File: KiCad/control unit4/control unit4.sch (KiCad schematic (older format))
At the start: 38 parts, among them J1 Conn_01x02_Female, J2 Conn_01x03_Female, J5 Conn_01x02_Female, U1 LM358, U2 LM358

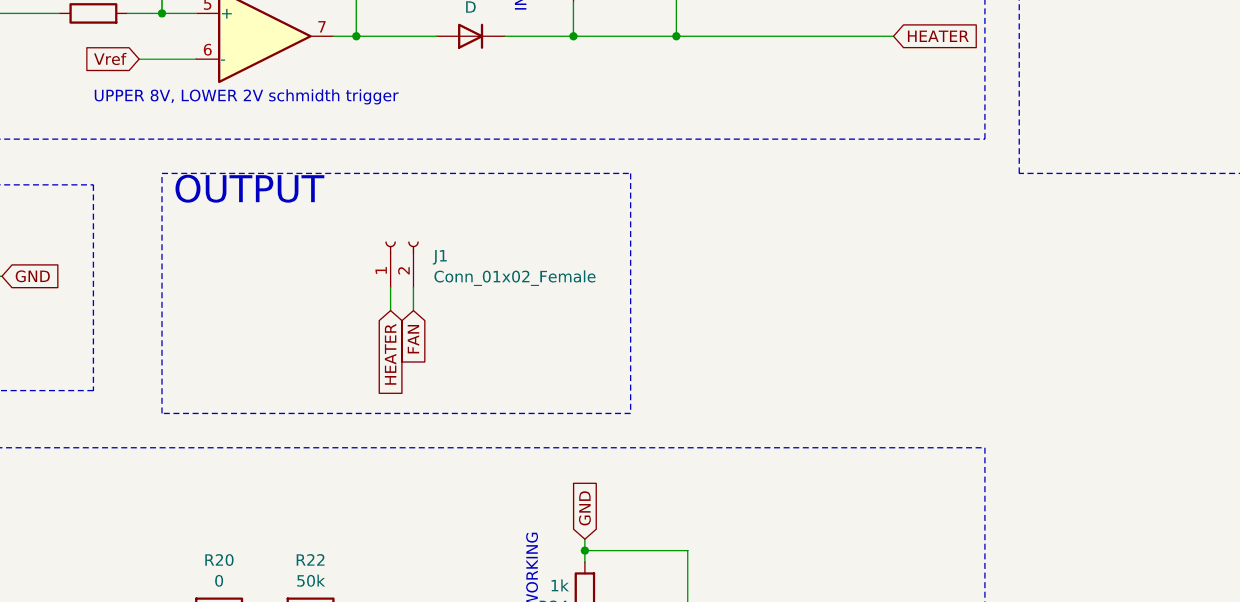
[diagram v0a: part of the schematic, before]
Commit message: Final report is finished
.
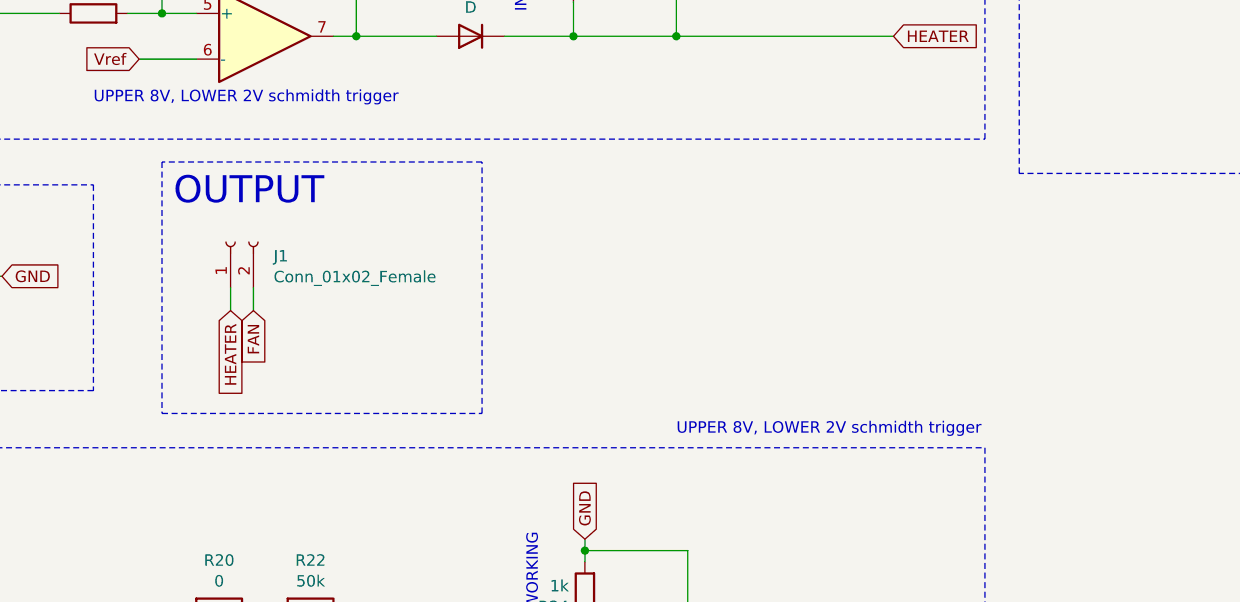
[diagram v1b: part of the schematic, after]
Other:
- moved on the sheet: J1
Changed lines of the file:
@@
 L Connector:Conn_01x02_Female J1
 U 1 1 6209D2C4
-P 4550 3100
-F 0 "J1" V 4488 2912 50  0000 R CNN
-F 1 "Conn_01x02_Female" V 4397 2912 50  0000 R CNN
-F 2 "TerminalBlock:TerminalBlock_Altech_AK300-2_P5.00mm" H 4550 3100 50  0001 C CNN
-F 3 "~" H 4550 3100 50  0001 C CNN
-	1    4550 3100
+P 3850 3100
+F 0 "J1" V 3788 2912 50  0000 R CNN
+F 1 "Conn_01x02_Female" V 3697 2912 50  0000 R CNN
+F 2 "TerminalBlock:TerminalBlock_Altech_AK300-2_P5.00mm" H 3850 3100 50  0001 C CNN
+F 3 "~" H 3850 3100 50  0001 C CNN
+	1    3850 3100
 	0    -1   -1   0
 $EndComp
 Wire Wire Line
-	4550 3300 4550 3400
+	3850 3300 3850 3400
 Wire Wire Line
-	4650 3400 4650 3300
-Text GLabel 4550 3400 3    50   Input ~ 0
+	3950 3400 3950 3300
+Text GLabel 3850 3400 3    50   Input ~ 0
 HEATER
-Text GLabel 4650 3400 3    50   Input ~ 0
+Text GLabel 3950 3400 3    50   Input ~ 0
 FAN
 Text Notes 5200 5350 1    50   ~ 0
@@
 Text Notes 5150 2100 1    50   ~ 0
 INDICATES HEATER IS WORKING
-Wire Notes Line
-	5600 2800 5600 3850
-Wire Notes Line
-	5600 3850 3550 3850
-Wire Notes Line
-	3550 3850 3550 2800
-Wire Notes Line
-	3550 2800 5600 2800
 Text Notes 3600 2950 0    118  ~ 0
 OUTPUT
@@
 Wire Wire Line
 	9050 2100 9050 2450
+Text Notes 5800 3950 0    50   ~ 0
+UPPER 8V, LOWER 2V schmidth trigger\n
+Wire Notes Line
+	3550 3850 4950 3850
+Wire Notes Line
+	4950 3850 4950 2750
+Wire Notes Line
+	4950 2750 3550 2750
+Wire Notes Line
+	3550 2750 3550 3850
 $EndSCHEMATC
